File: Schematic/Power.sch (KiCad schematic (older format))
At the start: 18 parts, among them U5 MCP73812T-420I-OT, U6 STC3100IST, U7 MIC5504-3.3YM5, U8 MIC5504-3.3YM5

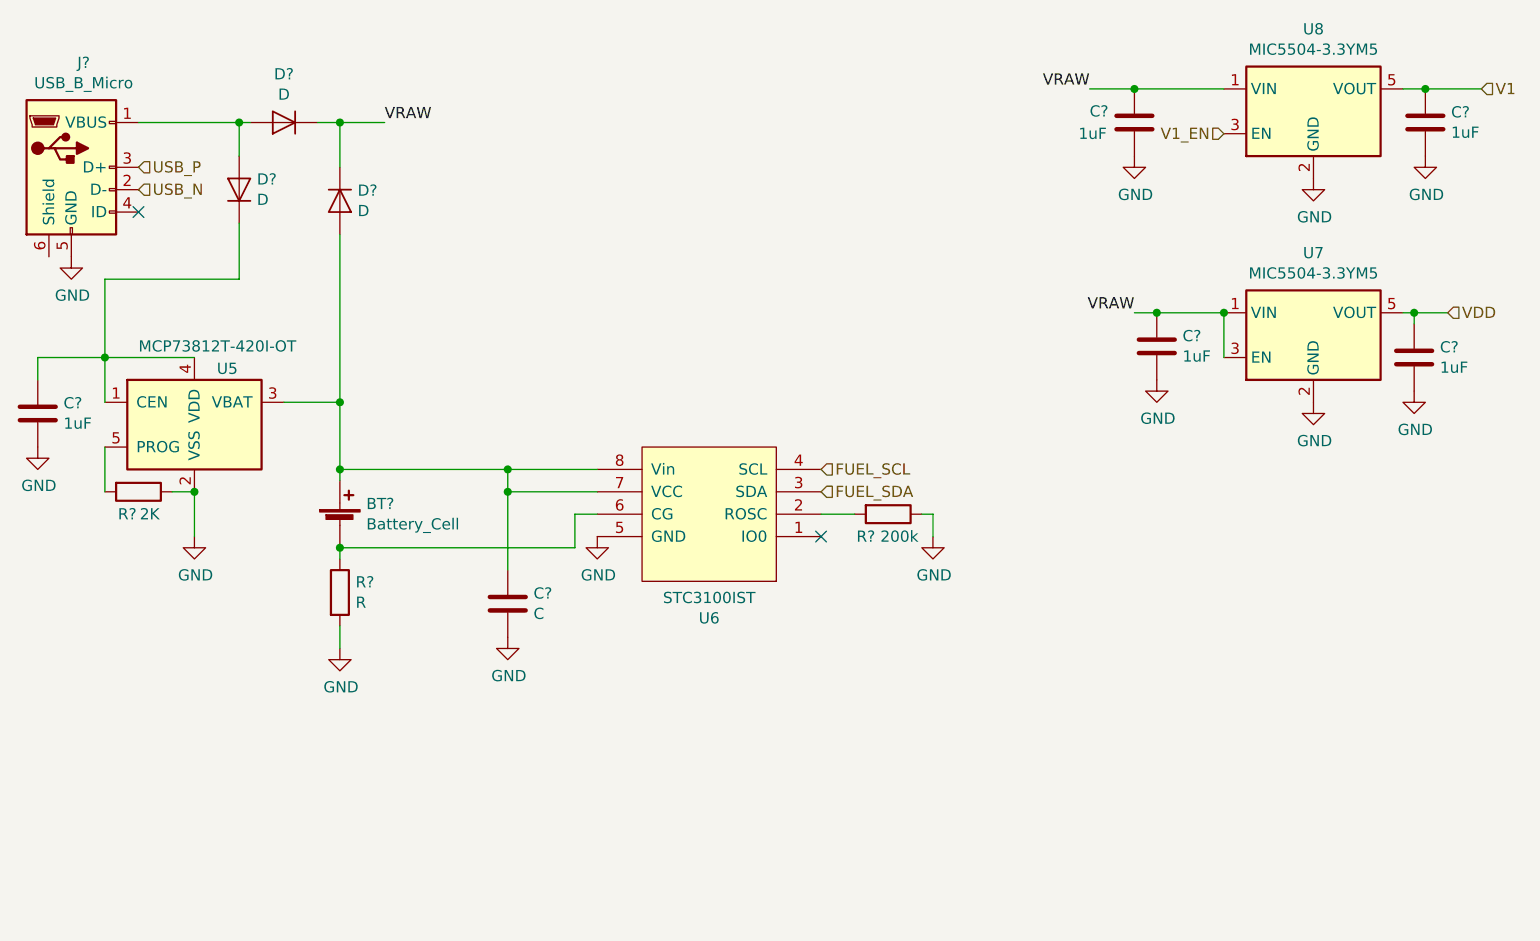
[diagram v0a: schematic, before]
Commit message: Add passives
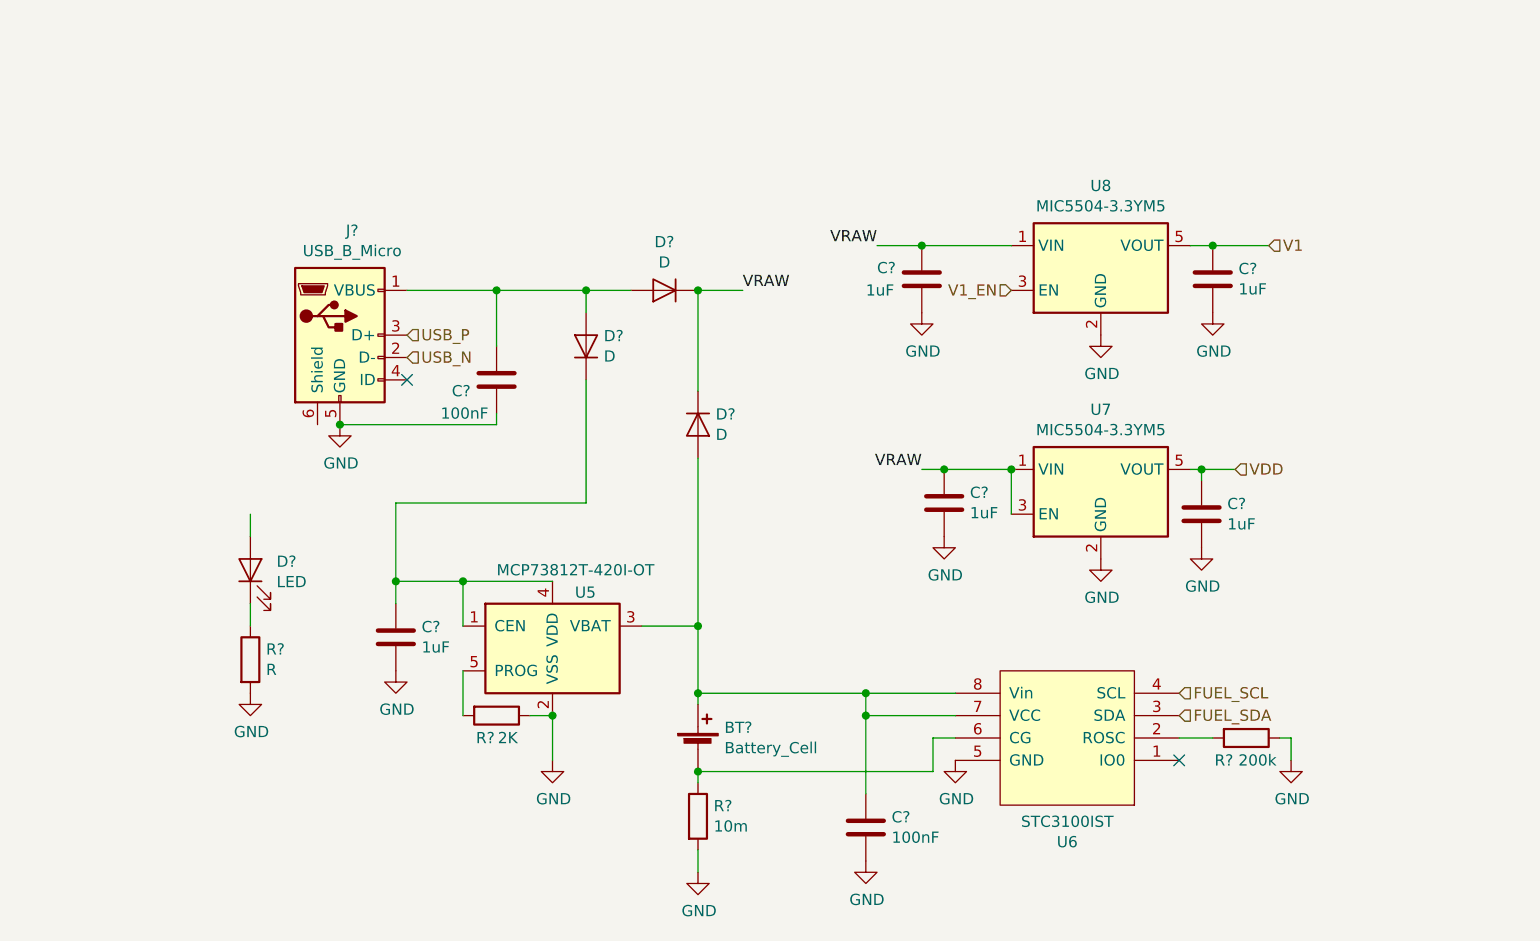
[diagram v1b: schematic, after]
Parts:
- added C?: 100nF, symbol Device:C
- added D?: LED, symbol Device:LED
- added R?: R, symbol Device:R
- C?: value C -> 100nF
- R?: value R -> 10m
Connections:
- net GND: now also C?.2, R?.2
- net at D?.2 (A), D?.2 (A), J?.1 (VBUS): now also C?.1
- new net: D?.1 (K), R?.1
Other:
- moved on the sheet: BT?, C?, D?, J?, R?, U5, U6, U7, U8
